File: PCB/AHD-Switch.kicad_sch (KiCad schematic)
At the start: 24 parts, among them J1 Conn_Coaxial, J2 Conn_Coaxial, J3 Conn_Coaxial, SW4 SW_Push, SW5 SW_Push, SW6 SW_Push, U1 TS5A63157DBV, U2 WEMOS_D1_mini

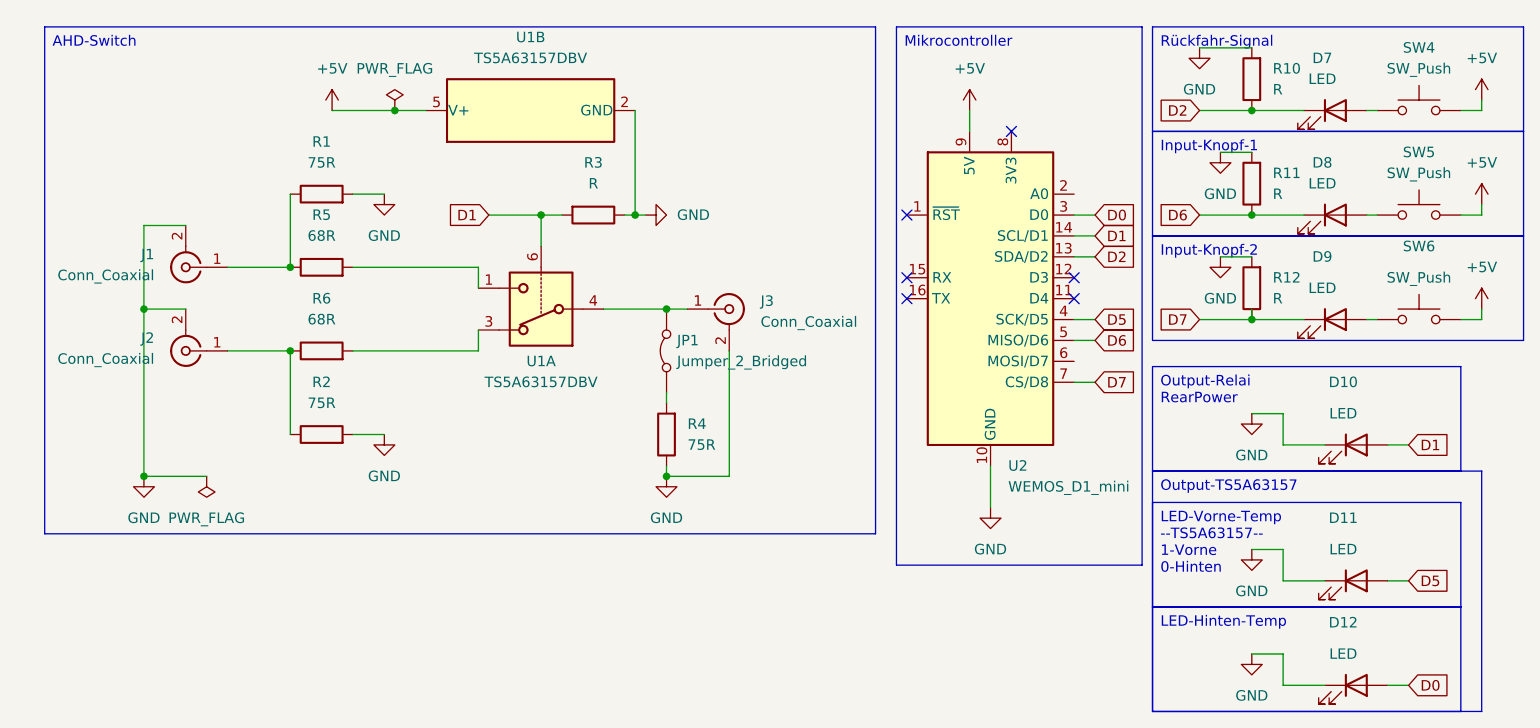
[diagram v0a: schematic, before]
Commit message: update§
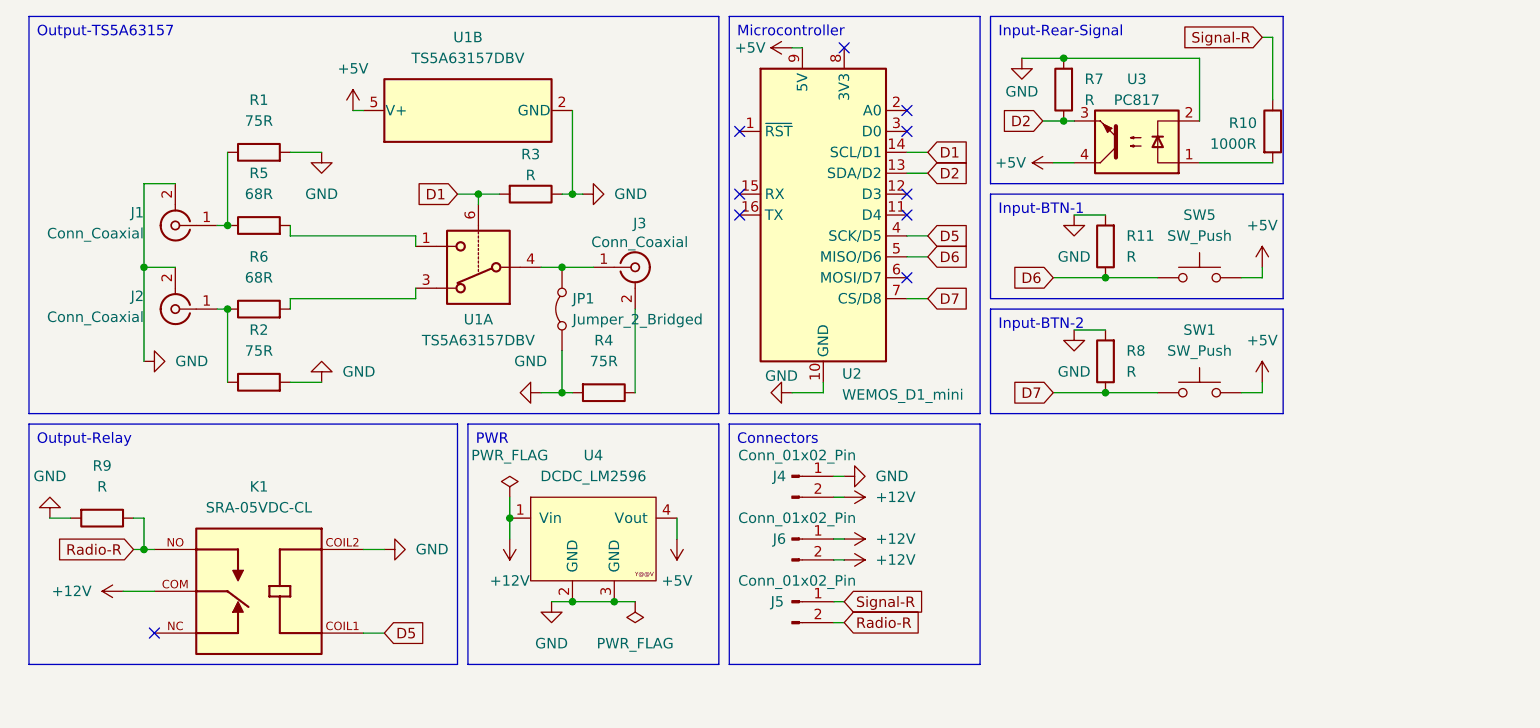
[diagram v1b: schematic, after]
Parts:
- removed D10, D11, D12, D7, D8, D9: LED, symbol Device:LED
- removed R12: R, symbol Device:R
- removed SW4, SW6: SW_Push, symbol Switch:SW_Push
- added J4, J5, J6: Conn_01x02_Pin, KF301-2P:HANDSON_KF301-2P, symbol Connector:Conn_01x02_Pin
- added K1: SRA-05VDC-CL, NightMeer:SRA-05VDC-CL, symbol NightMeer:SRA-05VDC-CL
- added R7, R8, R9: R, Resistor_THT:R_Axial_DIN0207_L6.3mm_D2.5mm_P10.16mm_Horizontal, symbol Device:R
- added SW1: SW_Push, KF301-2P:HANDSON_KF301-2P, symbol Switch:SW_Push
- added U3: PC817, Package_DIP:DIP-4_W7.62mm, symbol Isolator:PC817
- added U4: DCDC_LM2596, NightMeer:DCDC_LM2596, symbol NightMeer:DCDC_LM2596
- J1, J2, J3: footprint (none) -> NightMeer:CUI_RCJ-042
- JP1: footprint (none) -> NightMeer:Jumper_2.54mm
- R1, R11, R2, R3, R4, R5, R6: footprint (none) -> Resistor_THT:R_Axial_DIN0207_L6.3mm_D2.5mm_P10.16mm_Horizontal
- R10: value R -> 1000R; footprint (none) -> Resistor_THT:R_Axial_DIN0207_L6.3mm_D2.5mm_P10.16mm_Horizontal
- SW5: footprint (none) -> KF301-2P:HANDSON_KF301-2P
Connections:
- net +5V: now also SW1.2, U3.4, U4.4 (Vout)
- net D2: now also R7.1, U3.3; no longer R10.1
- net D5: now also K1.COIL1
- net D6: now also SW5.1
- net D7: now also R8.1, SW1.1
- net GND: now also JP1.1 (A), R4.2, J4.1 (Pin_1), K1.COIL2, R7.2, R8.2, R9.2, U3.2, U4.2 (GND), U4.3 (GND); no longer J3.2 (Ext), R10.2, R4.1
- net D0: no longer names the net of U2.3 (D0)
- new net: J3.2 (Ext), R4.1
- new net: R10.2, U3.1
- new net +12V: J4.2 (Pin_2), J6.1 (Pin_1), J6.2 (Pin_2), K1.COM, U4.1 (Vin)
- new net Radio-R: J5.2 (Pin_2), K1.NO, R9.1
- new net Signal-R: J5.1 (Pin_1), R10.1
- no-connect marks 6 -> 10
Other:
- moved on the sheet: J1, J2, J3, JP1, R1, R11, R2, R3, R4, R5, R6, SW5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

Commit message: Final PCB
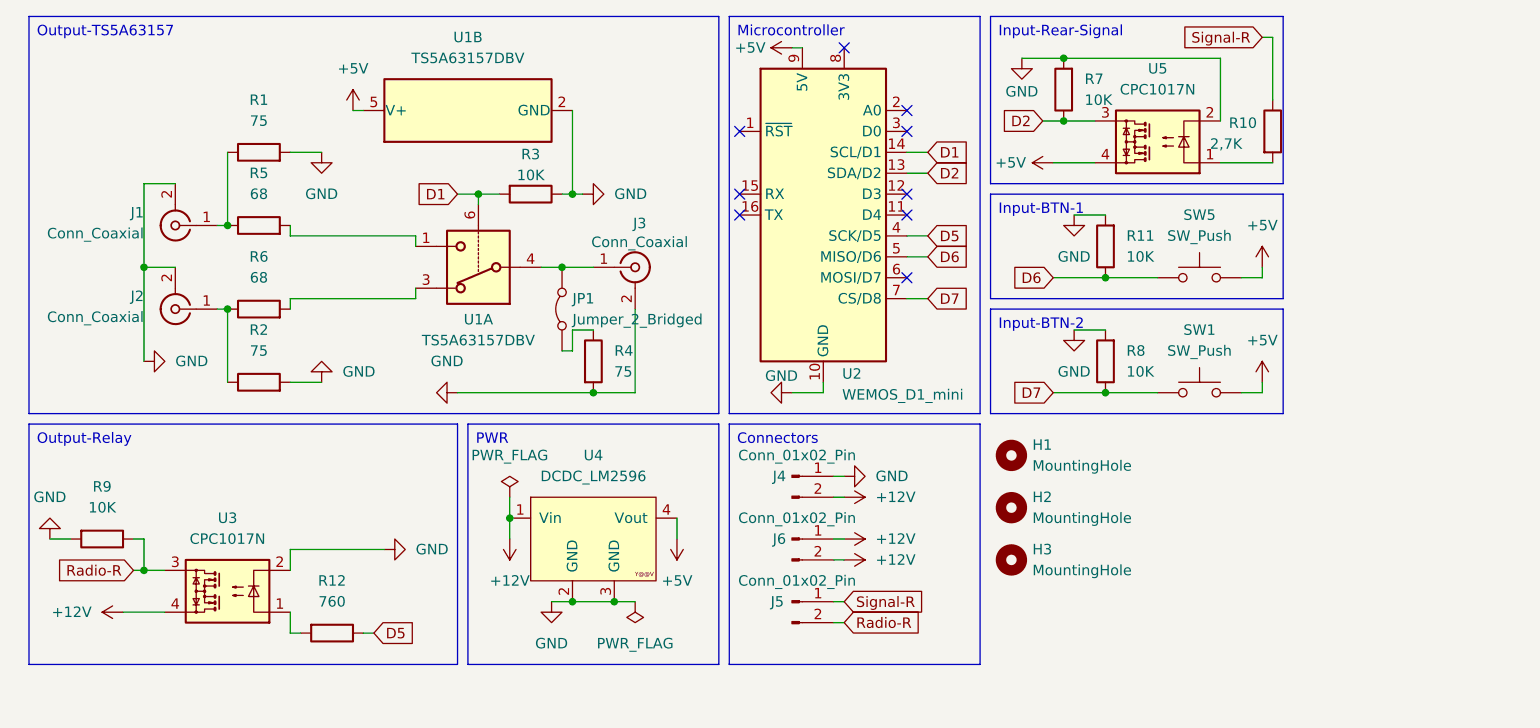
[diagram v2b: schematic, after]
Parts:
- removed K1: SRA-05VDC-CL, NightMeer:SRA-05VDC-CL, symbol NightMeer:SRA-05VDC-CL
- removed U3: PC817, Package_DIP:DIP-4_W7.62mm, symbol Isolator:PC817
- added H1, H2, H3: MountingHole, MountingHole:MountingHole_3.2mm_M3, symbol Mechanical:MountingHole
- added R12: 760, Resistor_THT:R_Axial_DIN0207_L6.3mm_D2.5mm_P10.16mm_Horizontal, symbol Device:R
- added U3, U5: CPC1017N, Package_SO:SOP-4_3.8x4.1mm_P2.54mm, symbol Relay_SolidState:CPC1017N
- R1, R2, R4: value 75R -> 75
- R10: value 1000R -> 2,7K
- R11, R3, R7, R8, R9: value R -> 10K
- R5, R6: value 68R -> 68
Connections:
- net +12V: now also U3.4
- net +5V: now also U5.4
- net D2: now also U5.3
- net D5: now also R12.1
- net GND: now also J3.2 (Ext), U3.2, U5.2; no longer JP1.1 (A)
- net Radio-R: now also U3.3
- net at R4.1: now also JP1.1 (A); no longer J3.2 (Ext)
- net at R10.2: now also U5.1
- new net: R12.2, U3.1
- no-connect marks 10 -> 9
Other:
- moved on the sheet: R4, R9
